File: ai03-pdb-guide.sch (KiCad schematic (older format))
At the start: 24 parts, among them SW1 SW_Push, U1 ATmega32U4-AU, Y1 16MHz

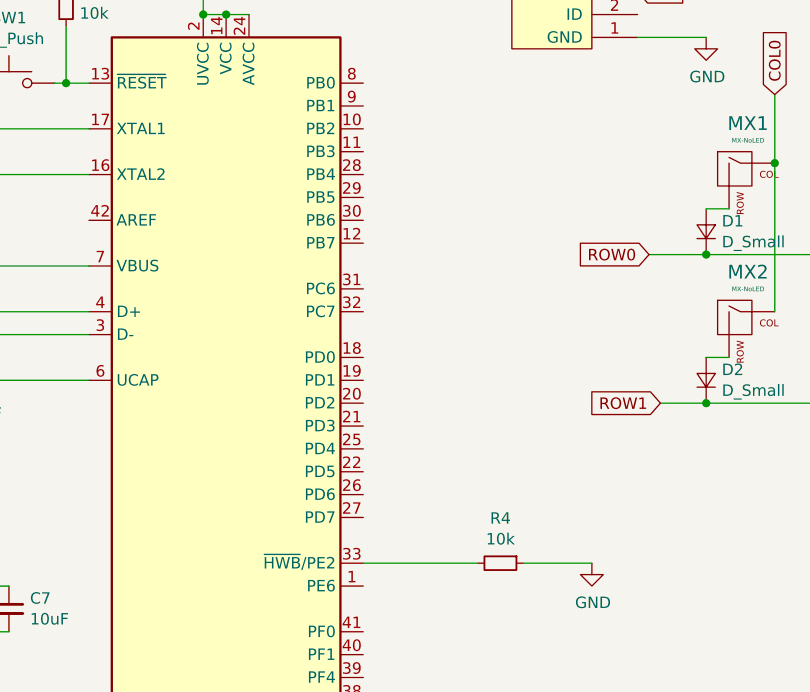
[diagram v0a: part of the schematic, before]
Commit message: maybe finished routing
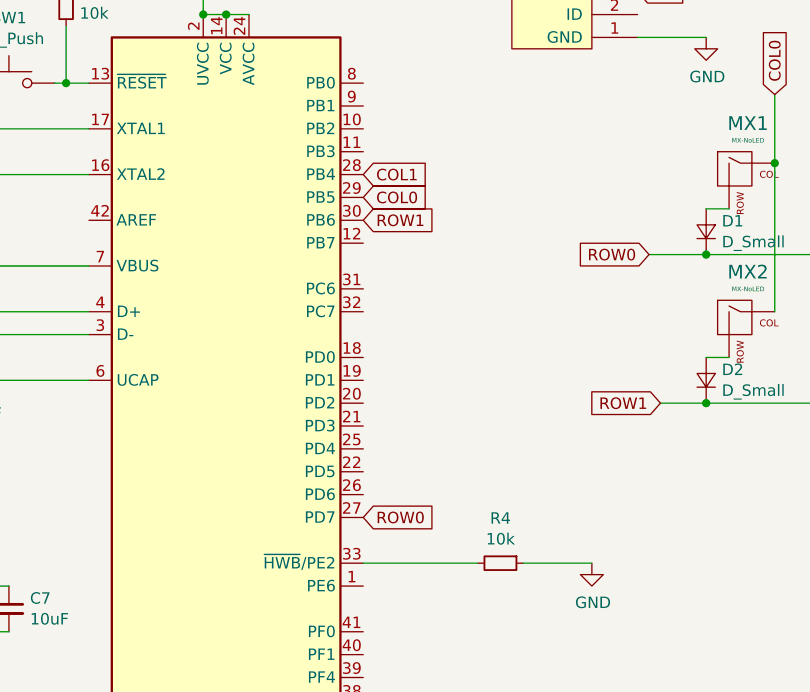
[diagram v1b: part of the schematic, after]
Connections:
- net COL0: now also U1.29 (PB5)
- net COL1: now also U1.28 (PB4)
- net ROW0: now also U1.27 (PD7)
- net ROW1: now also U1.30 (PB6)
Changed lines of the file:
@@
 EESchema Schematic File Version 4
+LIBS:ai03-pdb-guide-cache
 EELAYER 30 0
 EELAYER END
@@
 Text GLabel 5800 3150 0    50   Input ~ 0
 ROW1
+Text GLabel 4500 2250 2    50   Input ~ 0
+COL0
+Text GLabel 4500 2150 2    50   Input ~ 0
+COL1
+Text GLabel 4500 3650 2    50   Input ~ 0
+ROW0
+Text GLabel 4500 2350 2    50   Input ~ 0
+ROW1
 $EndSCHEMATC
